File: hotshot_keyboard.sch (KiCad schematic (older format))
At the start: 21 parts, among them J1 AVR-ISP-6, J2 USB_C_Receptacle_USB2.0, SW1 SW_Push, U1 ATmega32U4-AU, U2 PRTR5V0U2X, Y1 XTAL

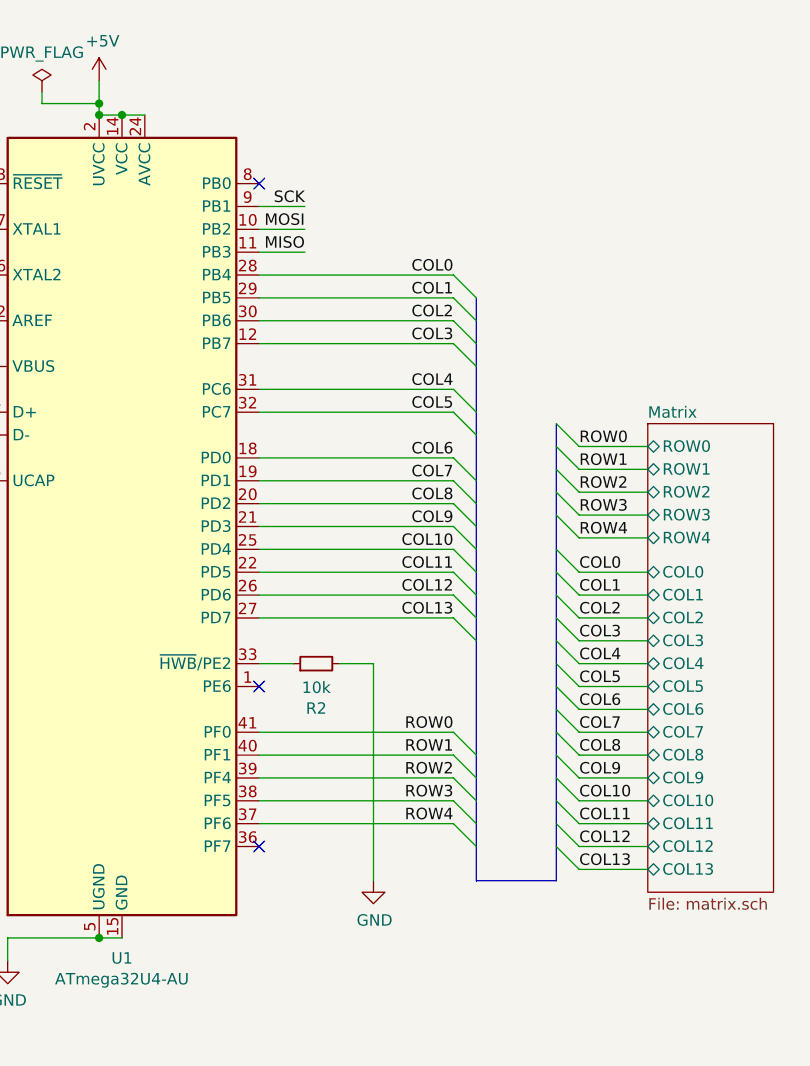
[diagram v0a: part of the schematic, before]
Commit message: reconfig schematics row/cols
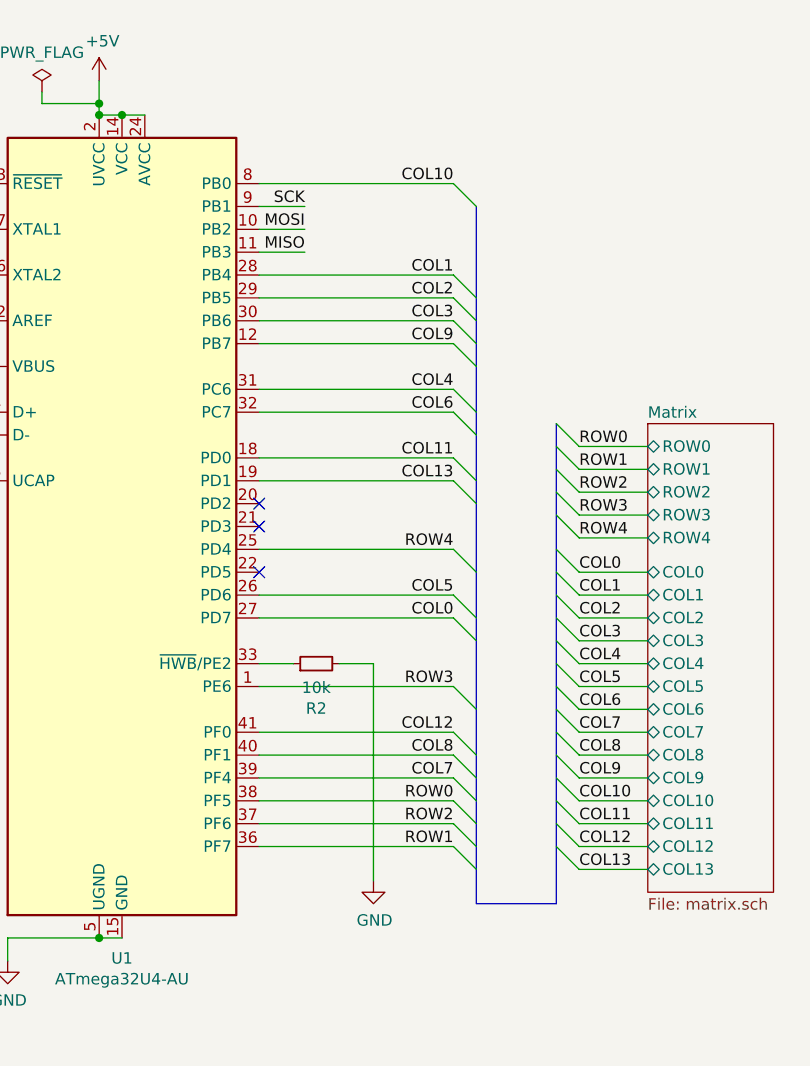
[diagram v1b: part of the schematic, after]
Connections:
- net COL0: now also U1.27 (PD7); no longer U1.28 (PB4)
- net COL1: now also U1.28 (PB4); no longer U1.29 (PB5)
- net COL10: now also U1.8 (PB0); no longer U1.25 (PD4)
- net COL11: now also U1.18 (PD0); no longer U1.22 (PD5)
- net COL12: now also U1.41 (PF0); no longer U1.26 (PD6)
- net COL13: now also U1.19 (PD1); no longer U1.27 (PD7)
- net COL2: now also U1.29 (PB5); no longer U1.30 (PB6)
- net COL3: now also U1.30 (PB6); no longer U1.12 (PB7)
- net COL5: now also U1.26 (PD6); no longer U1.32 (PC7)
- net COL6: now also U1.32 (PC7); no longer U1.18 (PD0)
- net COL7: now also U1.39 (PF4); no longer U1.19 (PD1)
- net COL8: now also U1.40 (PF1); no longer U1.20 (PD2)
- net COL9: now also U1.12 (PB7); no longer U1.21 (PD3)
- net ROW0: now also U1.38 (PF5); no longer U1.41 (PF0)
- net ROW1: now also U1.36 (PF7); no longer U1.40 (PF1)
- net ROW2: now also U1.37 (PF6); no longer U1.39 (PF4)
- net ROW3: now also U1.1 (PE6); no longer U1.38 (PF5)
- net ROW4: now also U1.25 (PD4); no longer U1.37 (PF6)
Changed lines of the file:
@@
 Wire Wire Line
 	6200 6800 6450 6800
+Text Label 7450 4500 2    50   ~ 0
+ROW0
+Text Label 7450 4700 2    50   ~ 0
+ROW1
+Text Label 7450 4600 2    50   ~ 0
+ROW2
+Text Label 7450 4000 2    50   ~ 0
+ROW3
+Text Label 7450 3400 2    50   ~ 0
+ROW4
+Text Label 7450 3700 2    50   ~ 0
+COL0
+Text Label 7450 2200 2    50   ~ 0
+COL1
+Text Label 7450 2300 2    50   ~ 0
+COL2
+Text Label 7450 2800 2    50   ~ 0
+COL6
+Text Label 7450 4400 2    50   ~ 0
+COL7
+Text Label 7450 4300 2    50   ~ 0
+COL8
+Text Label 7450 2500 2    50   ~ 0
+COL9
+Text Label 7450 1800 2    50   ~ 0
+COL10
+Text Label 7450 3000 2    50   ~ 0
+COL11
+Text Label 7450 2400 2    50   ~ 0
+COL3
 Text Label 7450 4200 2    50   ~ 0
-ROW0
-Text Label 7450 4300 2    50   ~ 0
-ROW1
-Text Label 7450 4400 2    50   ~ 0
-ROW2
-Text Label 7450 4500 2    50   ~ 0
-ROW3
-Text Label 7450 4600 2    50   ~ 0
-ROW4
-Text Label 7450 2200 2    50   ~ 0
-COL0
-Text Label 7450 2300 2    50   ~ 0
-COL1
-Text Label 7450 2400 2    50   ~ 0
-COL2
-Text Label 7450 3000 2    50   ~ 0
-COL6
+COL12
 Text Label 7450 3100 2    50   ~ 0
-COL7
-Text Label 7450 3200 2    50   ~ 0
-COL8
-Text Label 7450 3300 2    50   ~ 0
-COL9
-Text Label 7450 3400 2    50   ~ 0
-COL10
-Text Label 7450 3500 2    50   ~ 0
-COL11
-Text Label 7450 2500 2    50   ~ 0
-COL3
-Text Label 7450 3600 2    50   ~ 0
-COL12
-Text Label 7450 3700 2    50   ~ 0
 COL13
 $Sheet
@@
 	7450 3100 7550 3200
 Entry Wire Line
-	7450 3200 7550 3300
-Entry Wire Line
-	7450 3300 7550 3400
-Entry Wire Line
 	7450 3400 7550 3500
 Entry Wire Line
-	7450 3500 7550 3600
-Entry Wire Line
 	7450 3600 7550 3700
 Entry Wire Line
@@
 Wire Wire Line
 	7100 3900 7100 4850
-Text Label 7450 2800 2    50   ~ 0
+Text Label 7450 3600 2    50   ~ 0
 COL5
 Text Label 7450 2700 2    50   ~ 0
@@
 	6600 3600 7450 3600
 Wire Wire Line
-	7450 3500 6600 3500
-Wire Wire Line
 	6600 3400 7450 3400
 Wire Wire Line
-	7450 3300 6600 3300
-Wire Wire Line
-	6600 3200 7450 3200
-Wire Wire Line
 	7450 3100 6600 3100
-Wire Bus Line
-	7550 4850 7900 4850
-NoConn ~ 6600 1800
-NoConn ~ 6600 4000
-NoConn ~ 6600 4700
 Wire Wire Line
 	3700 7050 3850 7050
@@
 	2000 6300 2950 6300
 Connection ~ 2000 6300
-Wire Bus Line
-	7550 2300 7550 4850
-Wire Bus Line
-	7900 2850 7900 4850
 Text Label 2000 6300 0    50   ~ 0
 DD-
 Text Label 2000 6400 0    50   ~ 0
 DD+
+Wire Wire Line
+	6600 4700 7450 4700
+Entry Wire Line
+	7450 4700 7550 4800
+Wire Wire Line
+	6600 4000 7450 4000
+Entry Wire Line
+	7450 4000 7550 4100
+Wire Wire Line
+	6600 1800 7450 1800
+Entry Wire Line
+	7450 1800 7550 1900
+NoConn ~ 6600 3500
+NoConn ~ 6600 3300
+NoConn ~ 6600 3200
+Wire Bus Line
+	7550 4950 7900 4950
+Wire Bus Line
+	7550 1900 7550 4950
+Wire Bus Line
+	7900 2850 7900 4950
 $EndSCHEMATC
